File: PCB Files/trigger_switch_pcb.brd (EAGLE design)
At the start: 100 x 80 mm, 7 parts

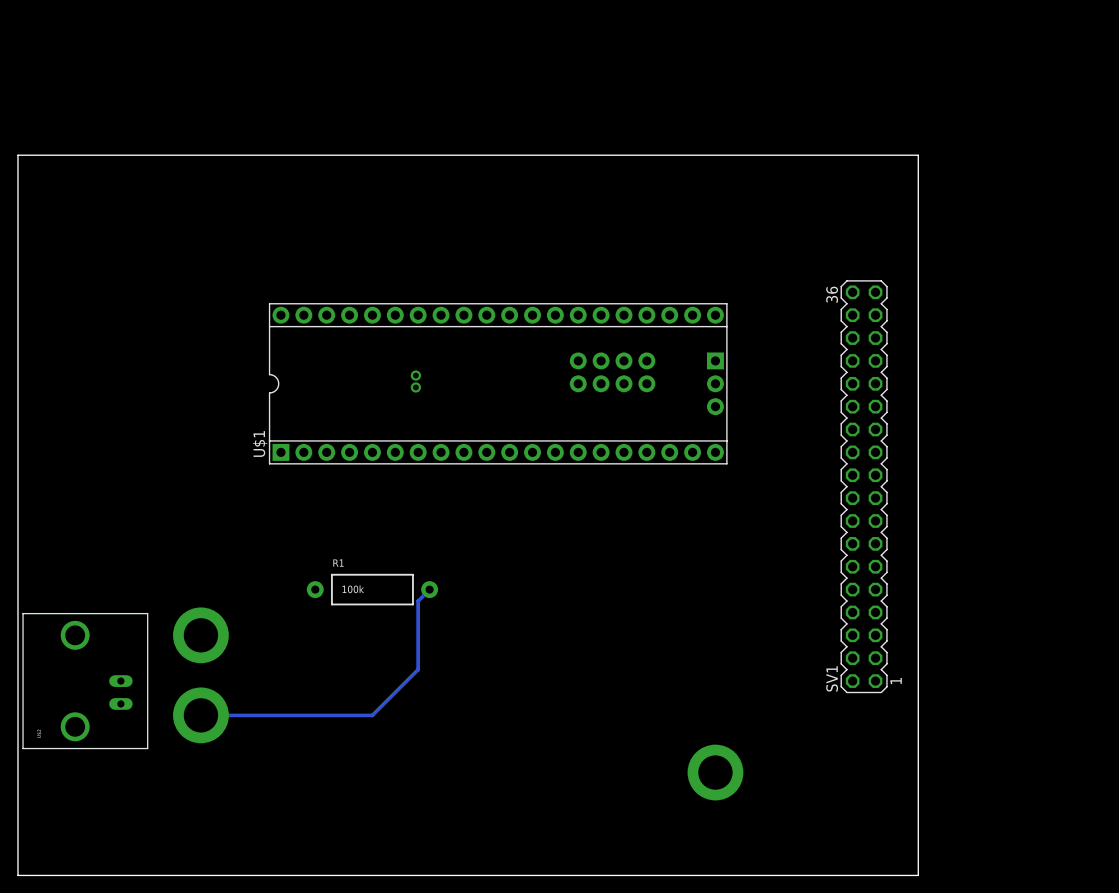
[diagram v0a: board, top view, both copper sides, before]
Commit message: update to wiring diagram
i think i have the board schematic done!   All grounds on the bottom,
all signals on the top
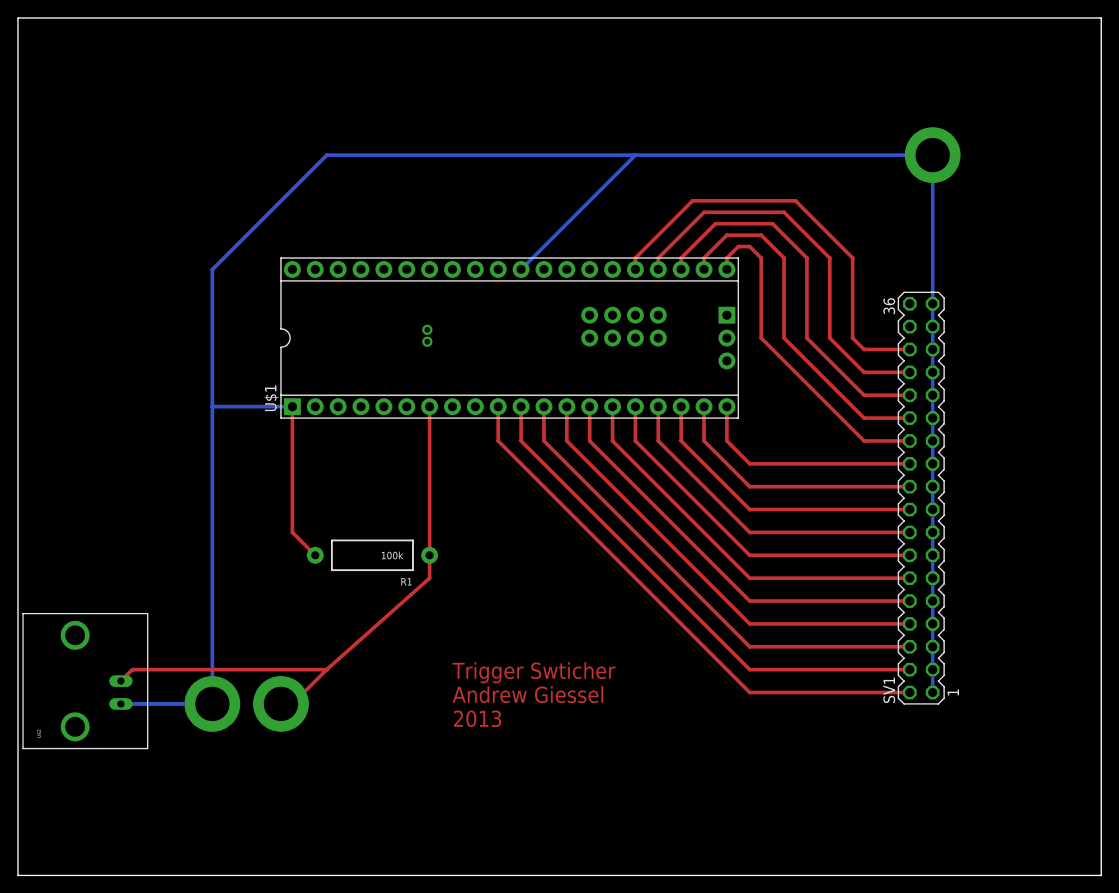
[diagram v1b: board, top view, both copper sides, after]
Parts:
- moved JP1 72.7 mm to (101.6, 80.0)
- moved JP2 11.7 mm to (29.2, 19.1)
- moved SV1 6.48 mm to (100.3, 41.9)
- moved U$1 5.24 mm to (54.6, 59.7)
- moved R1 3.81 mm to (39.4, 35.6), turned to 180 degrees
- moved JP3 1.80 mm to (21.6, 19.1)
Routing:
- net GND: track 35.7 -> 247.8 mm
- net TRIG: track 0.00 -> 64.3 mm
- net V1: track 0.00 -> 61.1 mm
- net V2: track 0.00 -> 57.5 mm
- net V3: track 0.00 -> 53.9 mm
- net V4: track 0.00 -> 50.3 mm
- net V5: track 0.00 -> 46.7 mm
- net V16: track 0.00 -> 46.4 mm
- net V15: track 0.00 -> 43.9 mm
- net V6: track 0.00 -> 43.1 mm
- net V14: track 0.00 -> 41.3 mm
- net V7: track 0.00 -> 39.6 mm
- net V13: track 0.00 -> 38.8 mm
- net V12: track 0.00 -> 36.3 mm
- net V8: track 0.00 -> 36.0 mm
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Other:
- board size 100 x 80 mm -> 120.3 x 95.2 mm
- board text added: "Trigger Swticher Andrew Giessel 2013"
